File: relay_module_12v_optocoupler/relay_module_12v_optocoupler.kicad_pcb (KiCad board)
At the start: 2 copper layers, 26.2 x 67.3 mm, 15 parts, among them J1 Conn_01x02_Pin, J2 Conn_01x03_Pin, K1 Relay_SPDT, Q1 BC337, U1 PC817

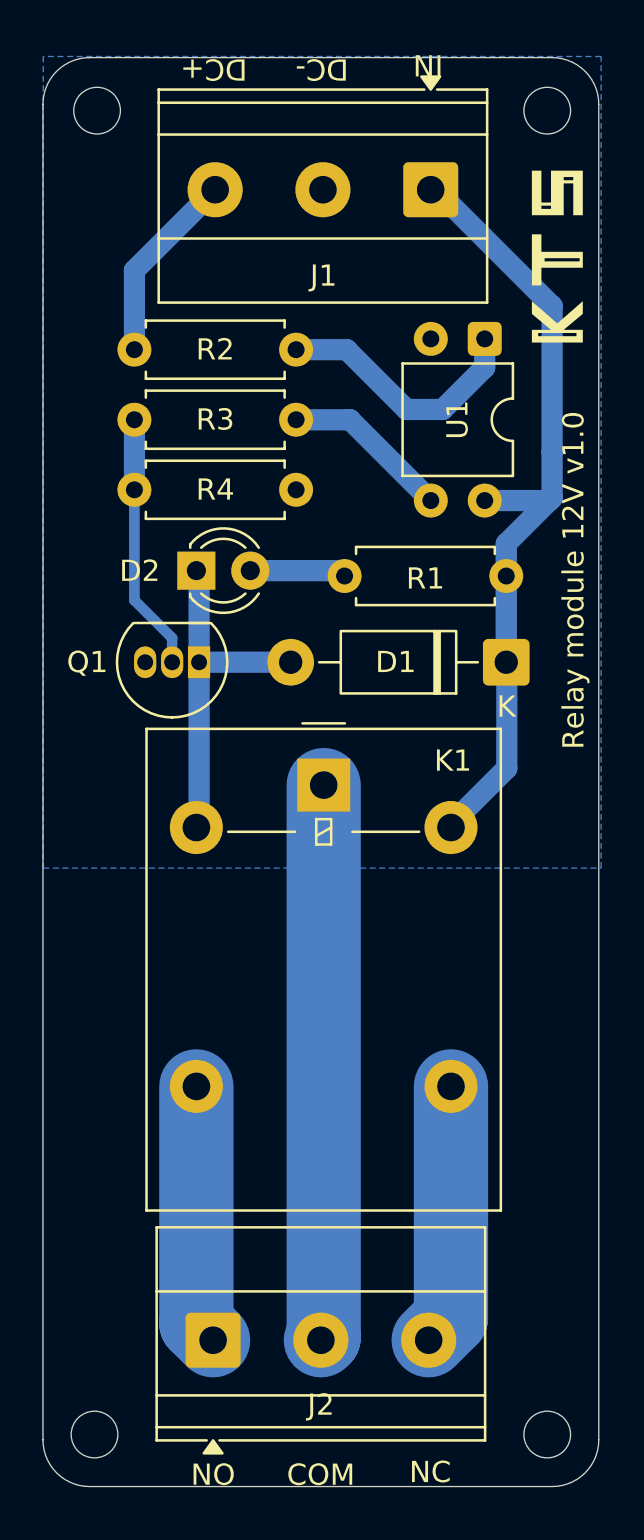
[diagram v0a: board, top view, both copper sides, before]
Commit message: v1.0.0
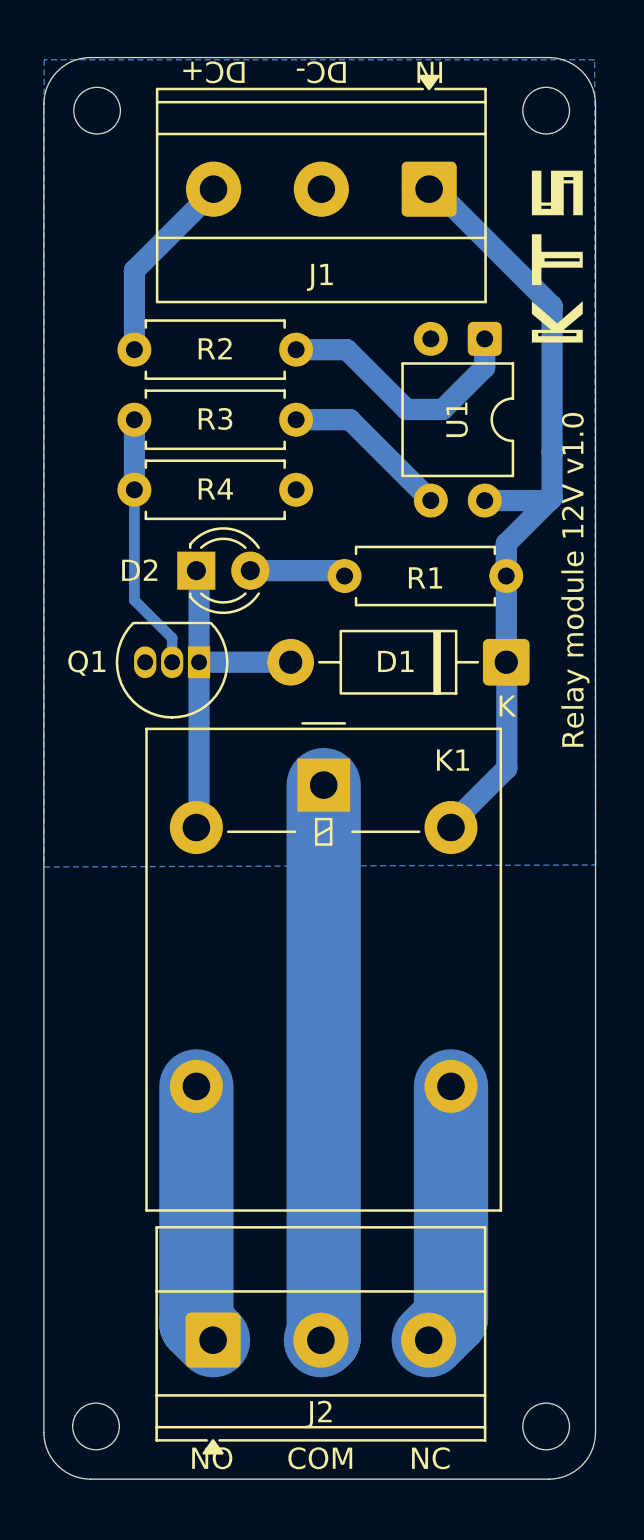
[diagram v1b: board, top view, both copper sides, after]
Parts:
- moved REF** 0.39 mm to (138.5, 137.4)
- moved REF** 0.38 mm to (159.7, 137.4)
- moved J1 0.08 mm to (154.2, 79.1)
- moved REF** 0.05 mm to (159.7, 75.4)
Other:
- board size 26.2 x 67.3 mm -> 26 x 67 mm
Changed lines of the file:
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@@
 			(outputformat 1)
 			(mirror no)
-			(drillshape 1)
+			(drillshape 0)
 			(scaleselection 1)
-			(outputdirectory "")
+			(outputdirectory "gerbers/")
 		)
 	)
@@
 	(footprint "MountingHole:MountingHole_2.2mm_M2"
 		(layer "F.Cu")
-		(at 159.766 137.795)
+		(at 159.7152 137.414)
 		(descr "Mounting Hole 2.2mm, M2, no annular, generated by kicad-footprint-generator mountinghole.py")
 		(tags "mountinghole M2")
@@
 	(footprint "MountingHole:MountingHole_2.2mm_M2"
 		(layer "F.Cu")
-		(at 159.766 75.4)
+		(at 159.7152 75.4)
 		(descr "Mounting Hole 2.2mm, M2, no annular, generated by kicad-footprint-generator mountinghole.py")
 		(tags "mountinghole M2")
@@
 	(footprint "TerminalBlock_Phoenix:TerminalBlock_Phoenix_MKDS-1,5-3-5.08_1x03_P5.08mm_Horizontal"
 		(layer "F.Cu")
-		(at 154.2746 79.1263 180)
+		(at 154.2 79.1 180)
 		(descr "Terminal Block Phoenix MKDS-1,5-3-5.08, 3 pins, pitch 5.08mm, size 15.2x9.8mm, drill diameter 1.3mm, pad diameter 2.6mm, http://www.farnell.com/datasheets/100425.pdf, script-generated using https://gitlab.com/kicad/libraries/kicad-footprint-generator/-/tree/master/scripts/TerminalBlock_Phoenix")
 		(tags "THT Terminal Block Phoenix MKDS-1,5-3-5.08 pitch 5.08mm size 15.2x9.8mm drill 1.3mm pad 2.6mm")
@@
 		(tags "THT Terminal Block Phoenix MKDS-1,5-3-5.08 pitch 5.08mm size 15.2x9.8mm drill 1.3mm pad 2.6mm")
 		(property "Reference" "J2"
-			(at 5.085 3.048 0)
+			(at 5.08 3.4036 0)
 			(layer "F.SilkS")
 			(effects
@@
 	(footprint "MountingHole:MountingHole_2.2mm_M2"
 		(layer "F.Cu")
-		(at 138.43 137.795)
+		(at 138.5 137.414)
 		(descr "Mounting Hole 2.2mm, M2, no annular, generated by kicad-footprint-generator mountinghole.py")
 		(tags "mountinghole M2")
@@
 		(layer "F.SilkS")
 	)
-	(gr_arc
-		(start 138.2 140.246)
-		(mid 136.644365 139.601635)
-		(end 136 138.046)
+	(gr_line
+		(start 159.8424 139.898)
+		(end 138.2424 139.898)
 		(stroke
 			(width 0.05)
@@
 		(layer "Edge.Cuts")
 	)
-	(gr_line
-		(start 159.996 140.246)
-		(end 138.2 140.246)
+	(gr_arc
+		(start 138.2424 139.898)
+		(mid 136.686765 139.253635)
+		(end 136.0424 137.698)
 		(stroke
 			(width 0.05)
@@
 		(layer "Edge.Cuts")
 	)
-	(gr_line
-		(start 136 138.046)
-		(end 136 75.1)
+	(gr_arc
+		(start 162.0424 137.698)
+		(mid 161.398035 139.253635)
+		(end 159.8424 139.898)
 		(stroke
 			(width 0.05)
@@
 		(layer "Edge.Cuts")
 	)
-	(gr_arc
-		(start 159.996 72.9)
-		(mid 161.551635 73.544365)
-		(end 162.196 75.1)
+	(gr_line
+		(start 136.0424 137.698)
+		(end 136.0424 75.098)
 		(stroke
 			(width 0.05)
@@
 	)
 	(gr_line
-		(start 138.2 72.9)
-		(end 159.996 72.9)
+		(start 138.2424 72.898)
+		(end 159.8424 72.898)
 		(stroke
 			(width 0.05)
@@
 		(layer "Edge.Cuts")
 	)
-	(gr_line
-		(start 162.196 75.1)
-		(end 162.196 138.046)
+	(gr_arc
+		(start 159.8424 72.898)
+		(mid 161.398035 73.542365)
+		(end 162.0424 75.098)
 		(stroke
 			(width 0.05)
@@
 		(layer "Edge.Cuts")
 	)
-	(gr_arc
-		(start 162.196 138.046)
-		(mid 161.551635 139.601635)
-		(end 159.996 140.246)
+	(gr_line
+		(start 162.0424 75.098)
+		(end 162.0424 137.698)
 		(stroke
 			(width 0.05)
@@
 	)
 	(gr_arc
-		(start 136 75.1)
-		(mid 136.644365 73.544365)
-		(end 138.2 72.9)
+		(start 136.0424 75.098)
+		(mid 136.686765 73.542365)
+		(end 138.2424 72.898)
 		(stroke
 			(width 0.05)
@@
 	)
 	(gr_text "DC-"
-		(at 149.1526 73.45 180)
+		(at 149.1526 73.5584 180)
 		(layer "F.SilkS")
 		(effects
@@
 	)
 	(gr_text "IN"
-		(at 154.1526 73.25 180)
+		(at 154.2288 73.5584 180)
 		(layer "F.SilkS")
 		(effects
@@
 	)
 	(gr_text "NO"
-		(at 144.018 139.7 0)
+		(at 143.95 138.95 0)
 		(layer "F.SilkS")
 		(effects
@@
 	)
 	(gr_text "NC"
-		(at 154.25 139.573 0)
+		(at 154.25 138.95 0)
 		(layer "F.SilkS")
 		(effects
@@
 	)
 	(gr_text "COM"
-		(at 149.098 139.7 0)
+		(at 149.098 138.95 0)
 		(layer "F.SilkS")
 		(effects
@@
 	)
 	(gr_text "DC+"
-		(at 144.0526 73.45 180)
+		(at 144.0526 73.5584 180)
 		(layer "F.SilkS")
 		(effects
@@
 		(polygon
 			(pts
-				(xy 136.0152 72.8472) (xy 136.0152 111.0972) (xy 162.306 111.0972) (xy 162.306 72.8472)
+				(xy 136.0576 73) (xy 136.0576 111.0464) (xy 162.0424 110.9492) (xy 162 73)
 			)
 		)
